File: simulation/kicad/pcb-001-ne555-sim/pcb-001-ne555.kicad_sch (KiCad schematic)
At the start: 14 parts, among them J1 +5 V / GND power input, U1 NE555D

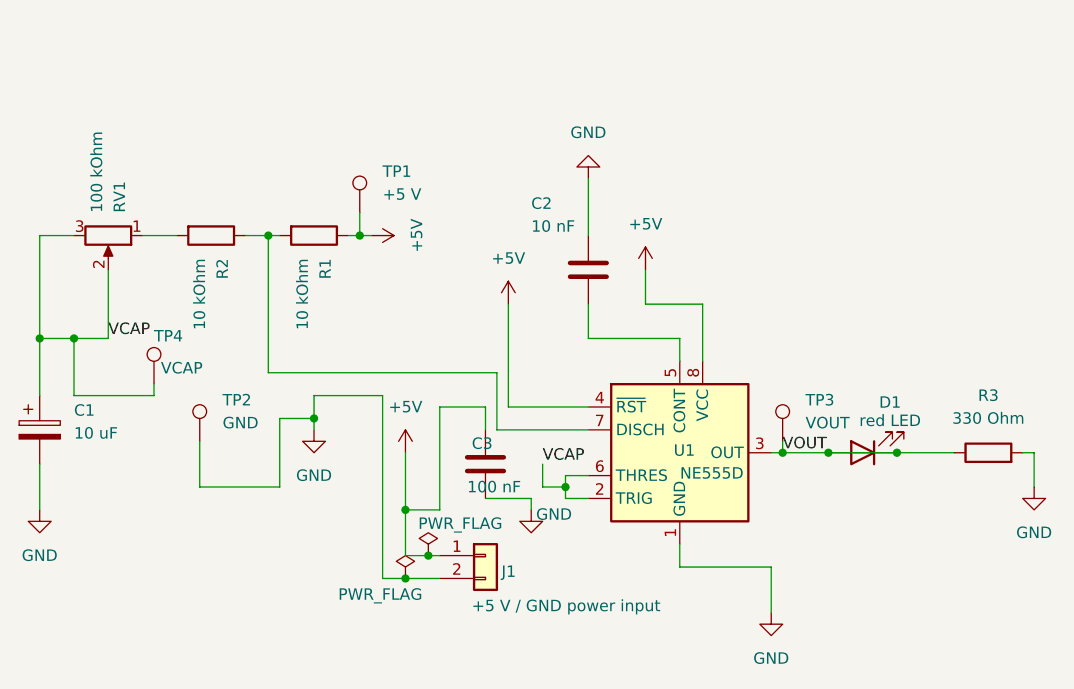
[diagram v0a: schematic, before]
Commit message: Update project files 2026-08-15 23:55:03
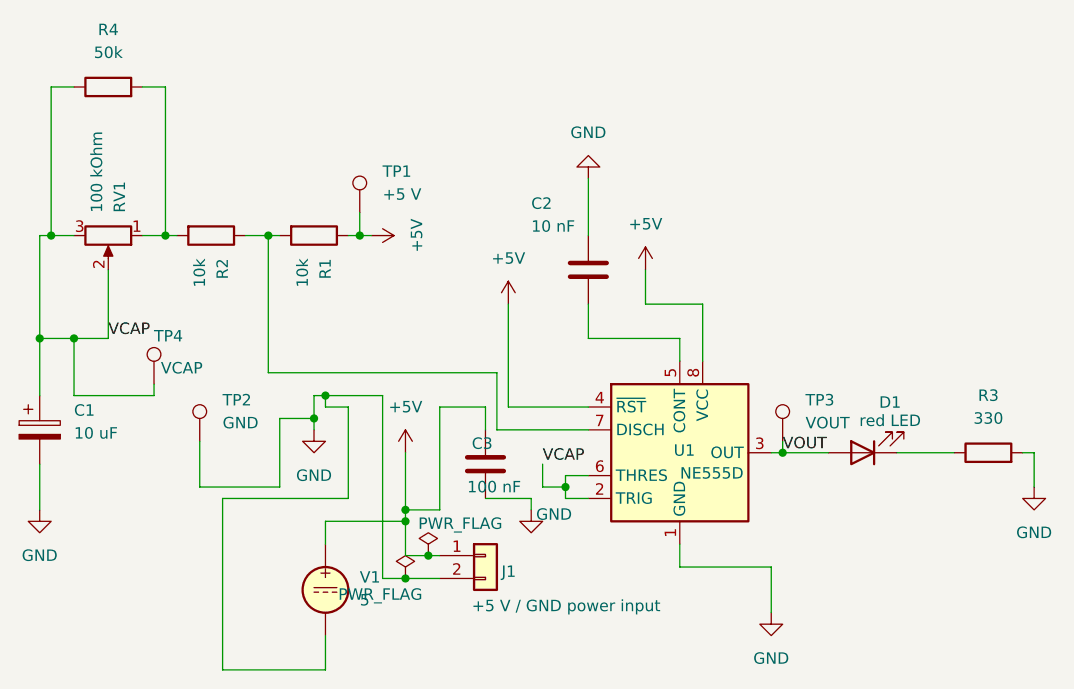
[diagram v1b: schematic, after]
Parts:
- added R4: 50k, symbol Device:R
- added V1: 5, symbol Simulation_SPICE:VDC
- R1, R2: value 10 kOhm -> 10k
- R3: value 330 Ohm -> 330
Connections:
- net +5V: now also V1.1
- net GND: now also V1.2
- net VCAP: now also R4.1
- net VOUT: no longer D1.1 (K), R3.1
- net at R2.2, RV1.1: now also R4.2
- new net: D1.1 (K), R3.1
